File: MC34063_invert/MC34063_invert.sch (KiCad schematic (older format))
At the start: 23 parts, among them J1 INPUT, J2 OUTPUT, Q1 BC557, U1 MC34063AP

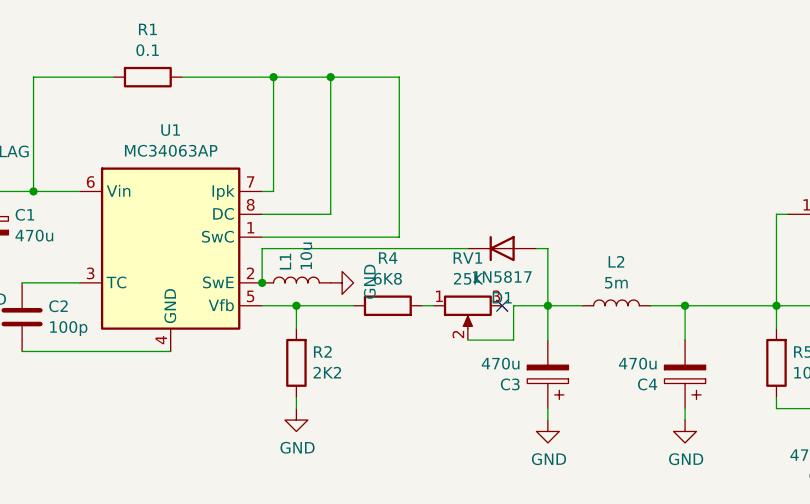
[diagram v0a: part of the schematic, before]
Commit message: Gerbers
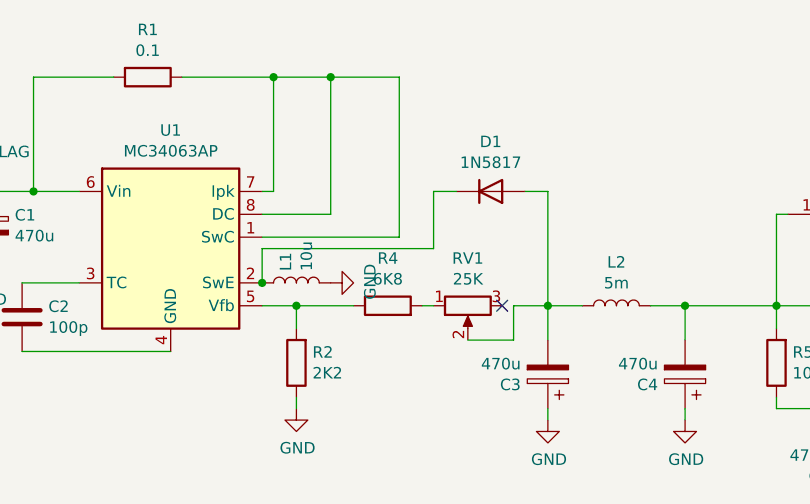
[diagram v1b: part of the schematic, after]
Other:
- moved on the sheet: D1
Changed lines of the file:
@@
 	4400 3000 4700 3000
-Wire Wire Line
-	4400 3100 5000 3100
 Wire Wire Line
 	3350 3300 3600 3300
@@
 F 3 "~" H 3350 3450 50  0001 C CNN
 	1    3350 3450
-	1    0    0    -1
-$EndComp
-$Comp
-L Device:D D1
-U 1 1 639830CC
-P 5450 3150
-F 0 "D1" H 5450 2933 50  0000 C CNN
-F 1 "1N5817" H 5450 3024 50  0000 C CNN
-F 2 "Diode_THT:D_A-405_P7.62mm_Horizontal" H 5450 3150 50  0001 C CNN
-F 3 "~" H 5450 3150 50  0001 C CNN
-	1    5450 3150
 	1    0    0    -1
 $EndComp
@@
 Wire Wire Line
 	5500 3550 5500 3400
-Wire Wire Line
-	5500 3400 5650 3400
 NoConn ~ 5450 3400
 $Comp
@@
 $EndComp
 Wire Wire Line
-	5650 3150 5650 3400
-Wire Wire Line
-	5600 3150 5650 3150
-Wire Wire Line
 	4400 3150 4400 3300
-Wire Wire Line
-	4400 3150 5300 3150
 Connection ~ 4400 3300
 Wire Wire Line
@@
 	0    -1   -1   0
 $EndComp
+Wire Wire Line
+	5500 3400 5650 3400
+Wire Wire Line
+	4400 3100 5000 3100
+$Comp
+L Device:D D1
+U 1 1 639830CC
+P 5400 2900
+F 0 "D1" H 5400 2683 50  0000 C CNN
+F 1 "1N5817" H 5400 2774 50  0000 C CNN
+F 2 "Diode_THT:D_A-405_P7.62mm_Horizontal" H 5400 2900 50  0001 C CNN
+F 3 "~" H 5400 2900 50  0001 C CNN
+	1    5400 2900
+	1    0    0    1
+$EndComp
+Wire Wire Line
+	5550 2900 5650 2900
+Wire Wire Line
+	5650 2900 5650 3400
+Wire Wire Line
+	5250 2900 5150 2900
+Wire Wire Line
+	5150 2900 5150 3150
+Wire Wire Line
+	5150 3150 4400 3150
 $EndSCHEMATC
